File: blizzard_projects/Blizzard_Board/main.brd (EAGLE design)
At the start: 67 x 80 mm, 81 parts, among them J1 XH_4POS_DEV, J2 XH_5POS_DEV, J3 XH_4POS_DEV, J4 XH_6POS_DEV, J5 XH_5POS_DEV, J6 XH_2POS_DEV, J7 XH_2POS_DEV, Q1 s8050(NPN), Q2 S8050(NPN), Q3 N2222, Q4 N2222, U1 USB_TO_UART_DEV, U2 BUCK_CONVERTER_DEV, U3 ESP_WROOM_32_DEV, U4 LAN8720_DEV, U5 MAX_485_DEV, X1 USB_CONN_DEV, X2 ETHERNET_DEV, Y1 50MHz

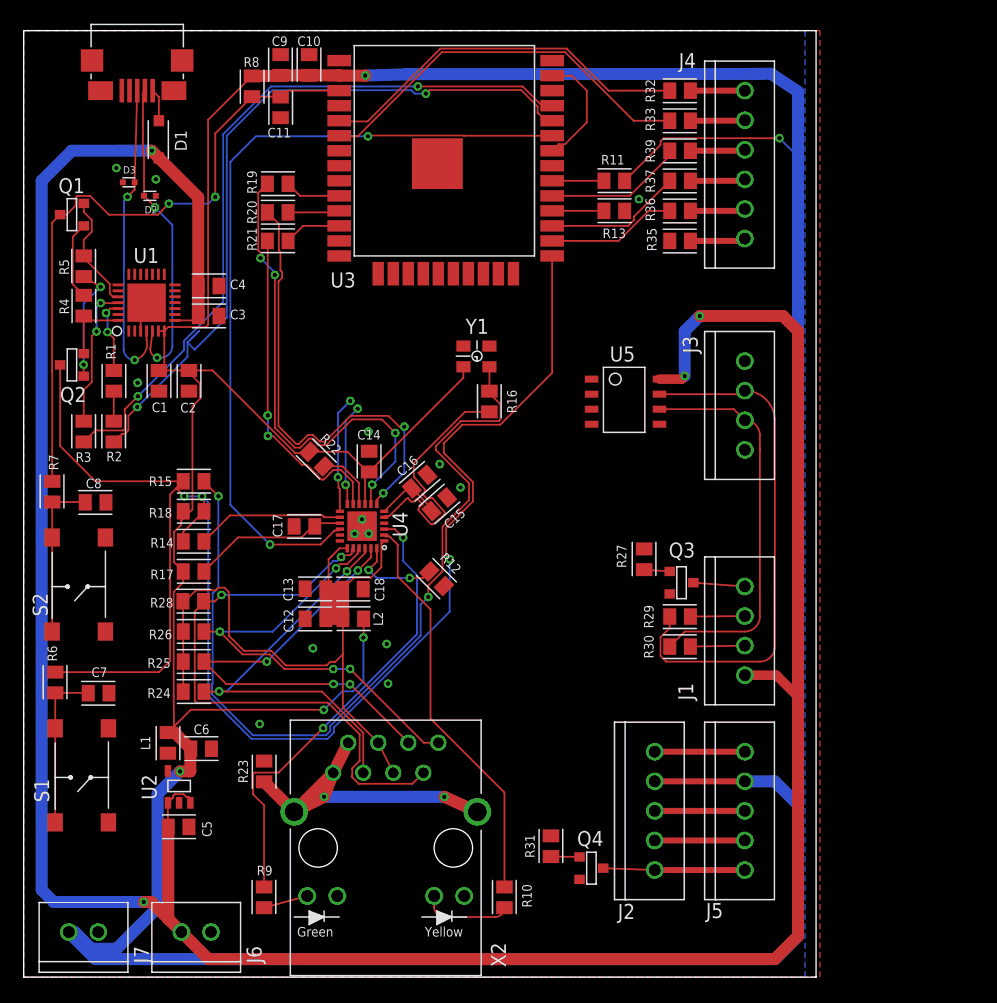
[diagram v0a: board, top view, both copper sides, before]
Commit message: finished tracing
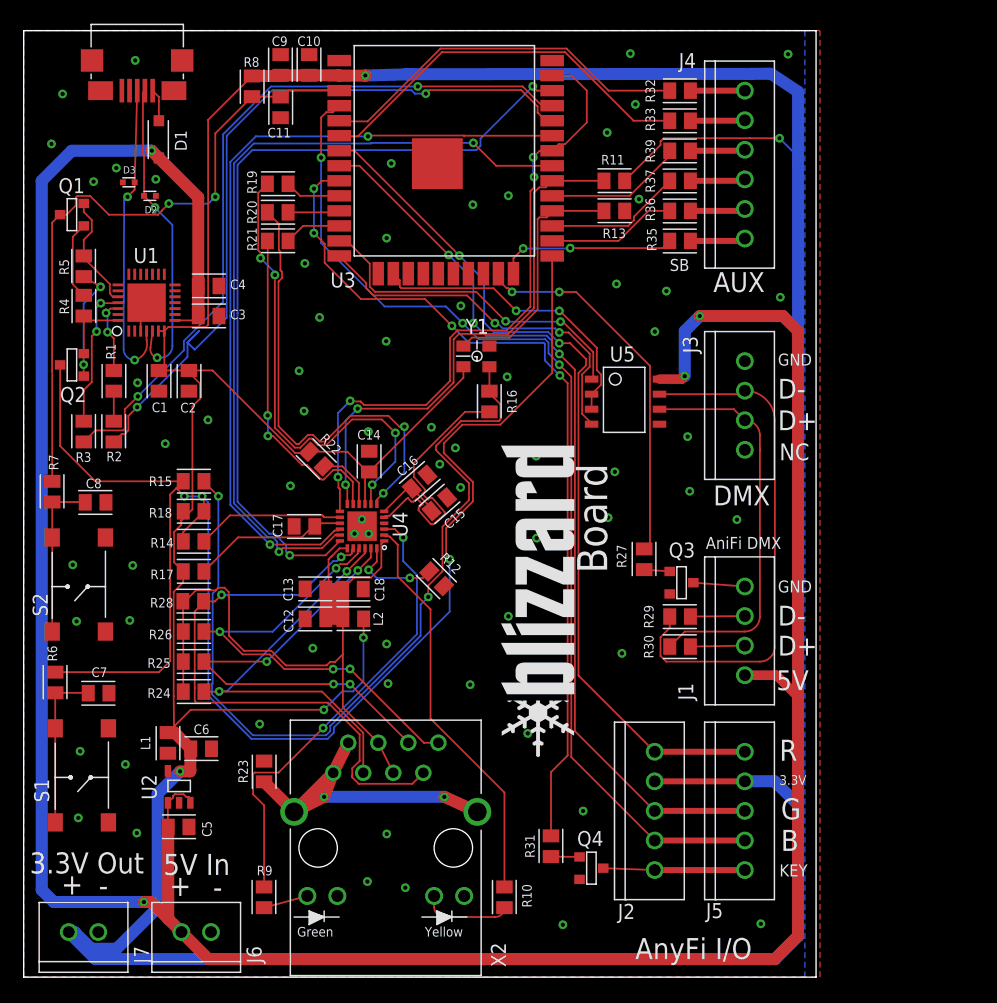
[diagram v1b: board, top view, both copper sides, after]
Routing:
- net IO36: track 7.62 -> 88.7 mm, vias 0 -> 3
- net IO33: track 0.00 -> 73.5 mm, vias 0 -> 4
- net IO22: track 0.00 -> 69.7 mm, vias 0 -> 2
- net IO32: track 7.62 -> 77.2 mm, vias 0 -> 3
- net IO19: track 0.00 -> 68.8 mm, vias 0 -> 2
- net IO35: track 7.62 -> 74.0 mm, vias 0 -> 2
- net IO23: track 19.9 -> 55.5 mm, vias 2 -> 4
- net IO18: track 12.9 -> 45.2 mm
- net IO15: track 0.00 -> 32.0 mm, vias 0 -> 2
- net IO12: track 0.00 -> 31.6 mm, vias 0 -> 2
- net IO14: track 0.00 -> 28.9 mm, vias 0 -> 2
- net IO13: track 0.00 -> 25.8 mm, vias 0 -> 2
- net IO17: track 4.38 -> 21.2 mm
- net IO2: track 0.00 -> 15.1 mm, vias 0 -> 2
- net GND: vias 14 -> 67
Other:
- board text added: "-... . . .--."
- board text added: "Board"

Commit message: v1 out to order
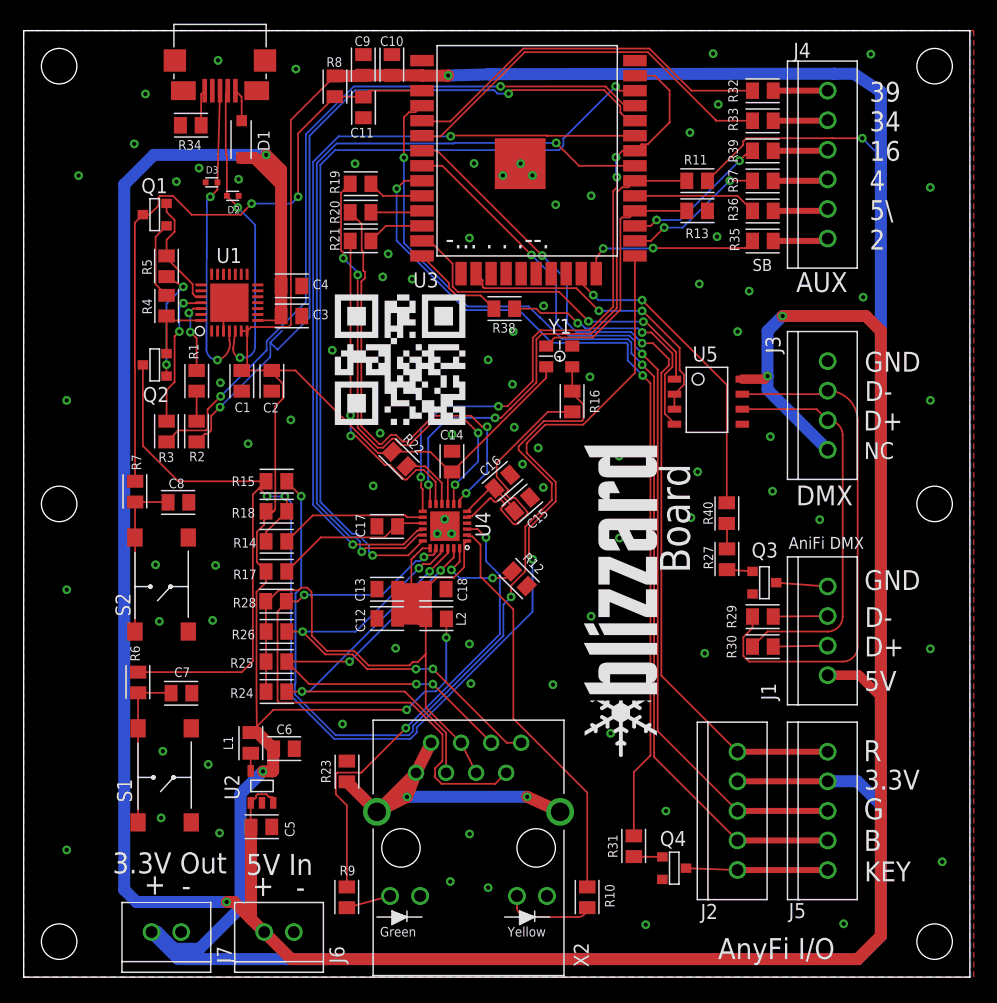
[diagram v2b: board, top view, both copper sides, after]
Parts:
- added R34, R38, R40: 0, blizzard_common_1:0805_PKG
- R4, R5: value 0805_RES_DEV -> 12K
- moved C8 7.00 mm to (12.2, 40.1)
- moved C1 7.00 mm to (18.4, 49.5)
- moved C10 7.00 mm to (31.1, 78.0)
- moved C11 7.00 mm to (28.7, 72.6)
- moved C14 7.00 mm to (36.2, 44.5)
- moved C15 7.00 mm to (42.8, 40.5)
- moved C16 7.00 mm to (41.1, 42.5)
- moved C17 7.00 mm to (29.9, 38.1)
- moved C18 7.00 mm to (35.7, 32.8)
- moved C3 7.00 mm to (23.5, 55.9)
- moved C4 7.00 mm to (23.5, 58.4)
- moved C6 7.00 mm to (22.9, 19.3)
- moved C7 7.00 mm to (12.5, 24.0)
- moved C9 7.00 mm to (28.7, 78.0)
- moved D1 7.00 mm to (18.4, 72.4)
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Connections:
- removed net N$31: U4.4
- new net N$13: R38.P$2, U3.IO12
- new net N$14: R40.P$2, U3.IO15
- net 5V: now also J3.P$4
- net GND: now also R34.P$2
- net IO12: now also R38.P$1; no longer U3.IO12
- net IO15: now also R40.P$1; no longer U3.IO15
- net IO16: now also R39.P$1; no longer R37.P$1
- net IO4: now also R37.P$1; no longer R36.P$1
- net IO5: now also R36.P$1; no longer R39.P$1
- net N$8: now also R34.P$1
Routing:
- net IO15: track 32.0 -> 2.85 mm, vias 2 -> 0
- net N$14: track 0.00 -> 26.6 mm, vias 0 -> 2
- net 5V: track 243.7 -> 257.2 mm
- net IO12: track 31.6 -> 21.5 mm
- net N$13: track 0.00 -> 8.18 mm
- net ETH_VDD: track 66.6 -> 73.2 mm
- net N$8: track 0.00 -> 3.05 mm
- net N$7: track 0.00 -> 1.49 mm
- net RXD0: track 64.7 -> 63.3 mm
- net IO5: track 11.8 -> 10.5 mm
- net IO4: track 11.0 -> 12.1 mm, vias 0 -> 2
- net IO23: track 55.5 -> 54.4 mm
- net IO16: track 11.7 -> 12.6 mm, vias 0 -> 2
- net IO18: track 45.2 -> 44.4 mm
- net 3.3V: track 363.3 -> 363.9 mm
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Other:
- board size 67 x 80 mm -> 80 x 80 mm
- board text added: "16"
- board text added: "2"
- board text added: "34"
- board text added: "39"
- board text added: "4"
- board text added: "5\"
- board text added: "Suite-E's Butt ->"

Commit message: waiting on first order
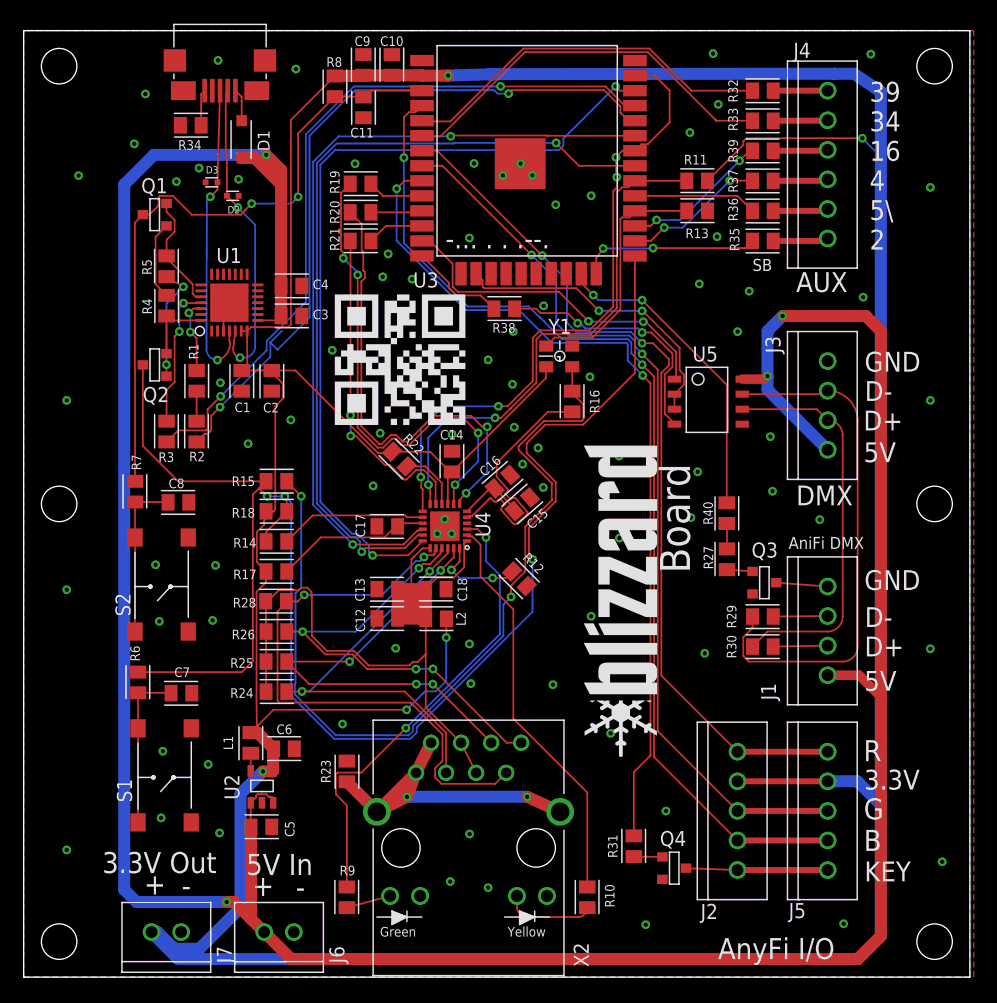
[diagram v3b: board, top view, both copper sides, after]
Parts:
- C12, C13, C14, C17: value 104 -> 0.1uF
- C15: value 0805_CAP_DEV -> 470pF
- C16: value 0805_CAP_DEV -> 1uF
- C18: value 0805_CAP_DEV -> 0.022uF
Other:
- board text removed: "NC"
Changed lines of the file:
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@@
 <grid distance="0.03" unitdist="mm" unit="mm" style="lines" multiple="1" display="yes" altdistance="0.005" altunitdist="mm" altunit="mm"/>
 <layers>
-<layer number="1" name="Top" color="4" fill="1" visible="yes" active="yes"/>
-<layer number="16" name="Bottom" color="1" fill="1" visible="yes" active="yes"/>
+<layer number="1" name="Top" color="9" fill="1" visible="yes" active="yes"/>
+<layer number="16" name="Bottom" color="3" fill="1" visible="no" active="yes"/>
 <layer number="17" name="Pads" color="2" fill="1" visible="yes" active="yes"/>
 <layer number="18" name="Vias" color="2" fill="1" visible="yes" active="yes"/>
 <layer number="19" name="Unrouted" color="6" fill="1" visible="no" active="yes"/>
 <layer number="20" name="Dimension" color="15" fill="1" visible="no" active="yes"/>
-<layer number="21" name="tPlace" color="7" fill="1" visible="no" active="yes"/>
-<layer number="22" name="bPlace" color="7" fill="1" visible="no" active="yes"/>
+<layer number="21" name="tPlace" color="7" fill="1" visible="yes" active="yes"/>
+<layer number="22" name="bPlace" color="7" fill="1" visible="yes" active="yes"/>
 <layer number="23" name="tOrigins" color="15" fill="1" visible="no" active="yes"/>
 <layer number="24" name="bOrigins" color="15" fill="1" visible="no" active="yes"/>
-<layer number="25" name="tNames" color="7" fill="1" visible="no" active="yes"/>
-<layer number="26" name="bNames" color="7" fill="1" visible="yes" active="yes"/>
+<layer number="25" name="tNames" color="7" fill="1" visible="yes" active="yes"/>
+<layer number="26" name="bNames" color="7" fill="1" visible="no" active="yes"/>
 <layer number="27" name="tValues" color="7" fill="1" visible="no" active="yes"/>
 <layer number="28" name="bValues" color="7" fill="1" visible="no" active="yes"/>
@@
 <wire x1="79.98" y1="80" x2="0" y2="80" width="0" layer="20"/>
 <wire x1="0" y1="80" x2="0" y2="0" width="0" layer="20"/>
-<text x="7.508" y="8.763" size="1.778" layer="21">3.3V Out</text>
+<text x="6.638" y="8.793" size="1.778" layer="21">3.3V Out</text>
 <text x="10.175" y="6.985" size="1.778" layer="21">+</text>
 <text x="13.35" y="6.858" size="1.778" layer="21">-</text>
@@
 <text x="64.658" y="36.195" size="1.016" layer="21">AniFi DMX</text>
 <text x="61.61" y="59.69" size="1.016" layer="21">SB</text>
-<text x="71.031" y="43.798" size="1.4224" layer="21">NC</text>
+<text x="71.001" y="43.528" size="1.6764" layer="21">5V</text>
 <rectangle x1="53.04855" y1="24.399871875" x2="54.04295625" y2="24.407240625" layer="21" rot="R90"/>
 <rectangle x1="53.291628125" y1="25.68155625" x2="53.799878125" y2="25.688925" layer="21" rot="R90"/>
@@
 <attribute name="NAME" x="29.59" y="71.787" size="0.8128" layer="25" rot="R180"/>
 </element>
-<element name="C12" library="blizzard_common_1" package="0805_PKG" value="104" x="29.865" y="30.317" smashed="yes">
+<element name="C12" library="blizzard_common_1" package="0805_PKG" value="0.1uF" x="29.865" y="30.317" smashed="yes">
 <attribute name="NAME" x="28.863" y="29.165" size="0.8128" layer="25" rot="R90"/>
 </element>
-<element name="C13" library="blizzard_common_1" package="0805_PKG" value="104" x="29.865" y="32.797" smashed="yes">
+<element name="C13" library="blizzard_common_1" package="0805_PKG" value="0.1uF" x="29.865" y="32.797" smashed="yes">
 <attribute name="NAME" x="28.833" y="31.745" size="0.8128" layer="25" rot="R90"/>
 </element>
-<element name="C14" library="blizzard_common_1" package="0805_PKG" value="104" x="36.21" y="44.45" smashed="yes" rot="R270">
+<element name="C14" library="blizzard_common_1" package="0805_PKG" value="0.1uF" x="36.21" y="44.45" smashed="yes" rot="R270">
 <attribute name="NAME" x="35.2" y="45.44" size="0.8128" layer="25"/>
 </element>
-<element name="C15" library="blizzard_common_1" package="0805_PKG" value="0805_CAP_DEV" x="42.7992375" y="40.545496875" smashed="yes" rot="R221.1">
+<element name="C15" library="blizzard_common_1" package="0805_PKG" value="470pF" x="42.7992375" y="40.545496875" smashed="yes" rot="R221.1">
 <attribute name="NAME" x="43.89755" y="39.71574375" size="0.8128" layer="25" rot="R221.1"/>
 </element>
-<element name="C16" library="blizzard_common_1" package="0805_PKG" value="0805_CAP_DEV" x="41.129503125" y="42.45955" smashed="yes" rot="R221.1">
+<element name="C16" library="blizzard_common_1" package="0805_PKG" value="1uF" x="41.129503125" y="42.45955" smashed="yes" rot="R221.1">
 <attribute name="NAME" x="39.907815625" y="44.169796875" size="0.8128" layer="25" rot="R221.1"/>
 </element>
-<element name="C17" library="blizzard_common_1" package="0805_PKG" value="104" x="29.86" y="38.1" smashed="yes">
+<element name="C17" library="blizzard_common_1" package="0805_PKG" value="0.1uF" x="29.86" y="38.1" smashed="yes">
 <attribute name="NAME" x="28.87" y="37.18" size="0.8128" layer="25" rot="R90"/>
 </element>
-<element name="C18" library="blizzard_common_1" package="0805_PKG" value="0805_CAP_DEV" x="35.705" y="32.797" smashed="yes" rot="R180">
+<element name="C18" library="blizzard_common_1" package="0805_PKG" value="0.022uF" x="35.705" y="32.797" smashed="yes" rot="R180">
 <attribute name="NAME" x="36.673" y="33.745" size="0.8128" layer="25" rot="R270"/>
 </element>

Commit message: sent 1st order
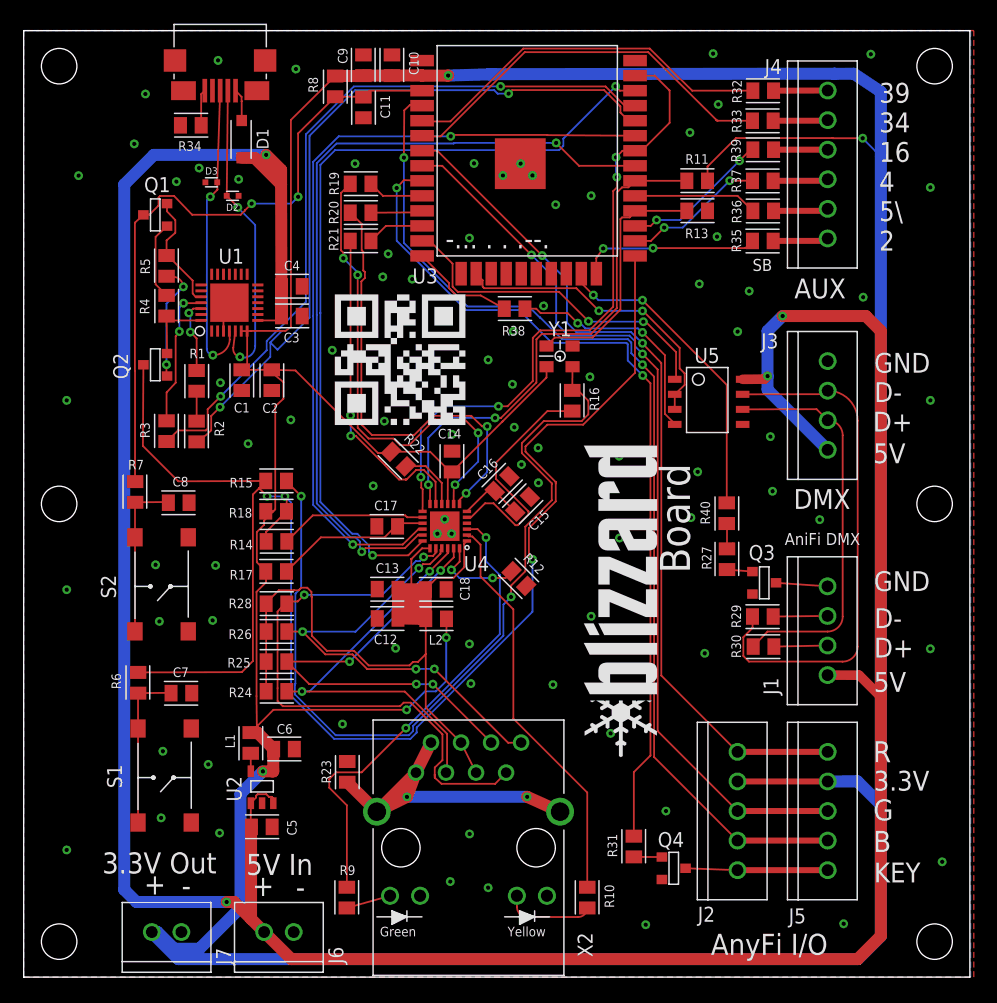
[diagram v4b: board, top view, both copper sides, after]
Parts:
- moved U3 12.7 mm to (42.7, 69.8)
- moved X2 8.31 mm to (37.6, 10.9)
- moved J4 6.24 mm to (68.0, 68.7)
- moved J2 5.01 mm to (60.3, 14.0)
- moved J5 5.01 mm to (68.0, 14.0)
- moved S2 4.58 mm to (11.7, 33.2)
- moved S1 4.55 mm to (11.9, 17.0)
- moved X1 4.01 mm to (16.6, 77.5)
- moved J3 3.75 mm to (68.0, 48.3)
- moved J1 3.74 mm to (68.0, 29.3)
- moved U5 3.49 mm to (57.9, 48.6)
- moved U1 2.83 mm to (17.4, 57.0)
- moved U4 2.27 mm to (35.6, 38.1)
- moved U2 1.63 mm to (20.2, 16.1)
- moved D1 1.56 mm to (18.4, 70.8)
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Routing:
- net IO12: track 21.5 -> 19.6 mm
- net N$32: track 22.2 -> 20.6 mm
- net N$34: track 39.3 -> 38.1 mm
- net IO35: track 74.0 -> 73.0 mm
- net N$13: track 8.18 -> 8.88 mm
- net CLK50: track 71.7 -> 72.3 mm
- net N$35: track 41.2 -> 40.6 mm
- net LED1: track 39.2 -> 39.8 mm
- net D+: track 26.3 -> 25.7 mm

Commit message: REV 1.2
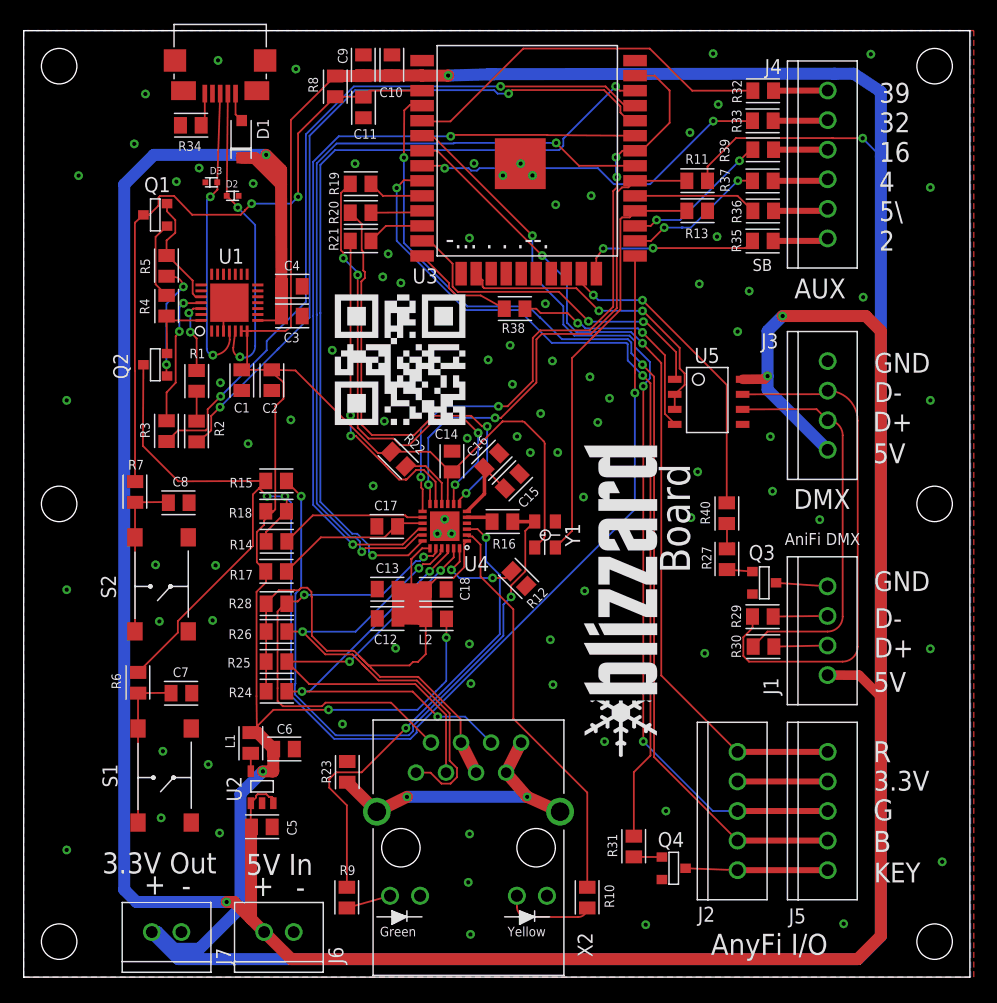
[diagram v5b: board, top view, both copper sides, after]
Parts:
- moved Y1 15.1 mm to (44.1, 37.4), turned to 90 degrees
- moved R16 11.8 mm to (40.5, 38.5), turned to 180 degrees
- moved C15 2.14 mm to (41.3, 41.9)
- moved C16 2.14 mm to (39.6, 43.7)
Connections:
- new net NC: J2.P$2, J5.P$2
- net 3.3V: no longer J2.P$2, J5.P$2
- net IO32: now also R33.P$1; no longer J2.P$3, J5.P$3
- net IO34: now also J2.P$3, J5.P$3; no longer R33.P$1
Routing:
- net IO34: track 33.4 -> 80.7 mm, vias 0 -> 3
- net IO32: track 77.2 -> 31.1 mm
- net N$32: track 20.6 -> 2.28 mm
- net CLK50: track 72.3 -> 54.2 mm
- net IO17: track 21.2 -> 36.8 mm
- net TXN: track 49.5 -> 38.3 mm
- net IO0: track 132.8 -> 123.9 mm
- net NC: track 0.00 -> 7.62 mm
- net 3.3V: track 364.3 -> 358.7 mm
- net N$37: track 29.3 -> 25.1 mm
- net ETH_VDD: track 72.9 -> 77.0 mm
- net TXP: track 38.6 -> 41.8 mm, vias 4 -> 2
- net RXD0: track 63.3 -> 60.8 mm
- net VDDCR: track 5.96 -> 7.04 mm
- net RXN: track 35.9 -> 36.6 mm, vias 2 -> 3
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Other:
- board text added: "32"
- board text added: "VER 1.2"
- board text removed: "34"
